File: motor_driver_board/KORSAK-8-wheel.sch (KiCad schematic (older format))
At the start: 24 parts, among them J1 Screw_Terminal_01x04, J2 Conn_01x02_Male, J3 Screw_Terminal_01x06, J4 Screw_Terminal_01x04, M1 Motor_DC, M2 Motor_DC, M3 Motor_DC, M4 Motor_DC, M5 Motor_DC, M6 Motor_DC, M7 Motor_DC, M8 Motor_DC, U1 L293D, U2 L293D, U3 L293D, U4 L293D

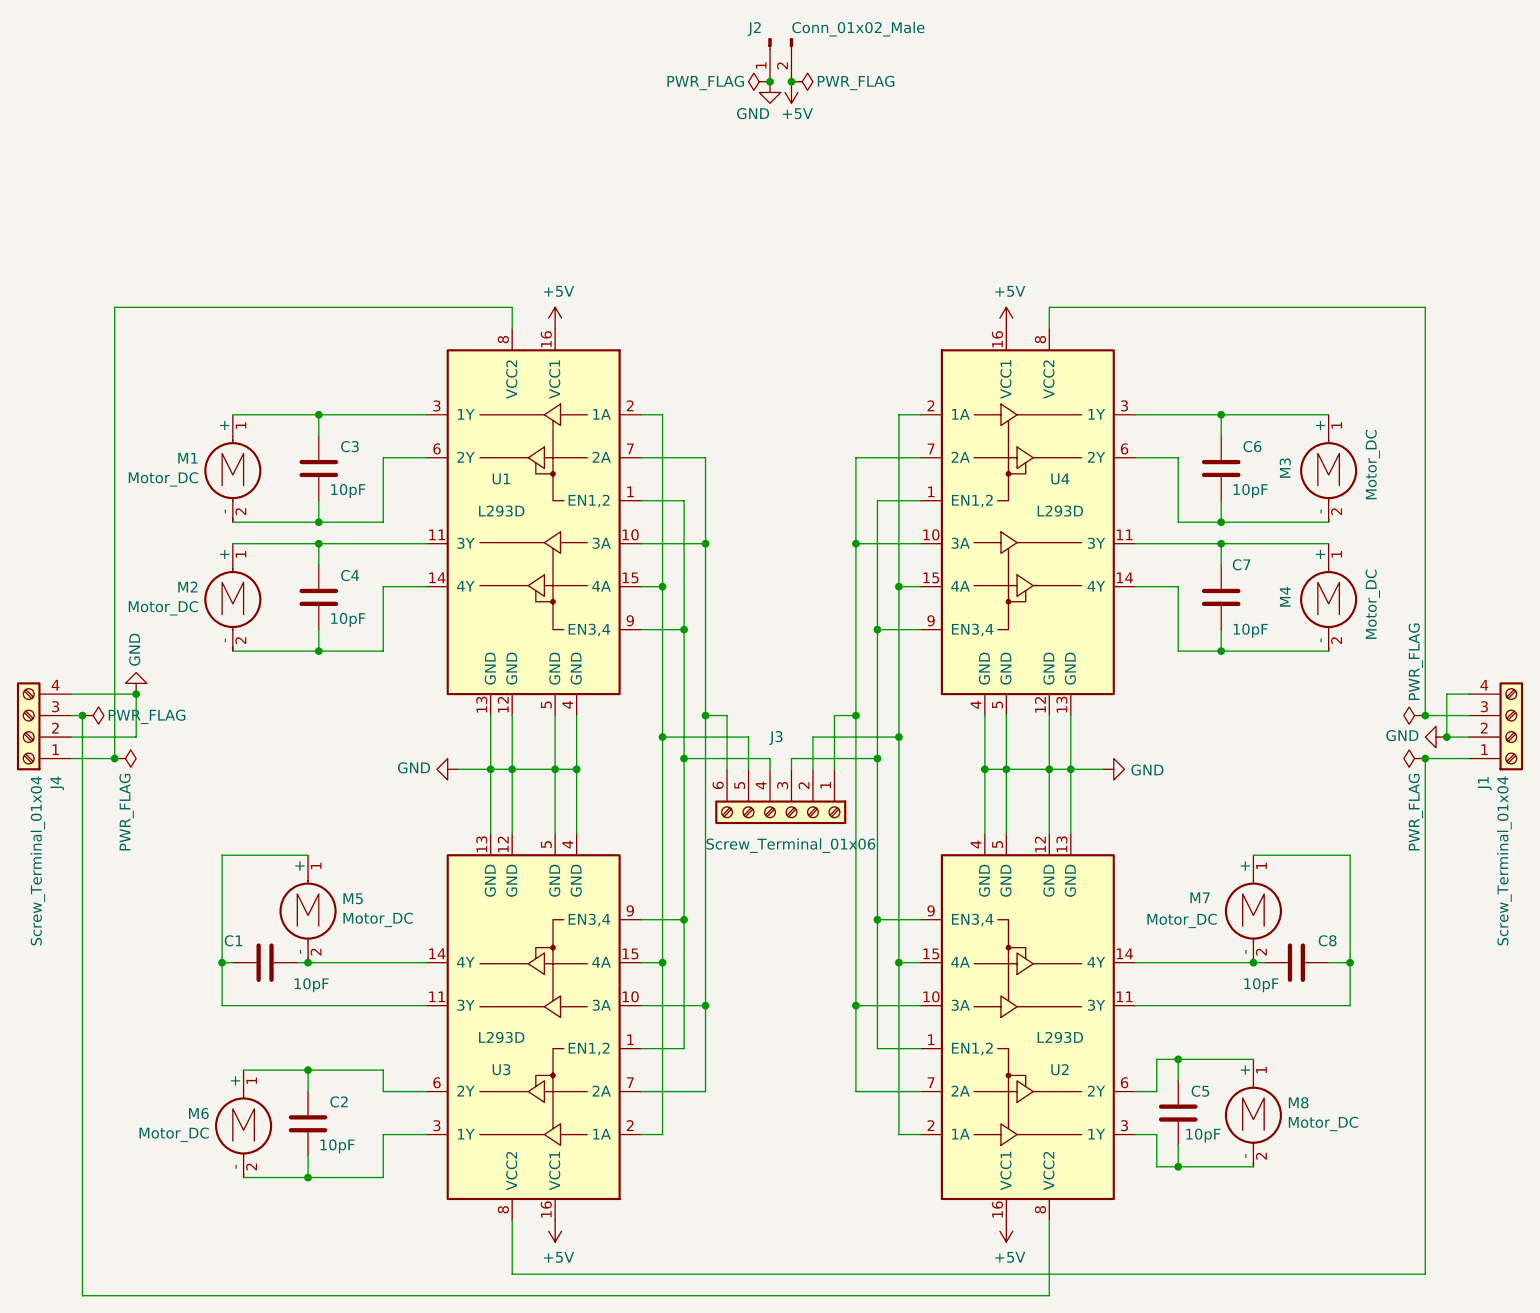
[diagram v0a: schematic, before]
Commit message: Откат прошлого коммита, т.к. это незаконченная версия
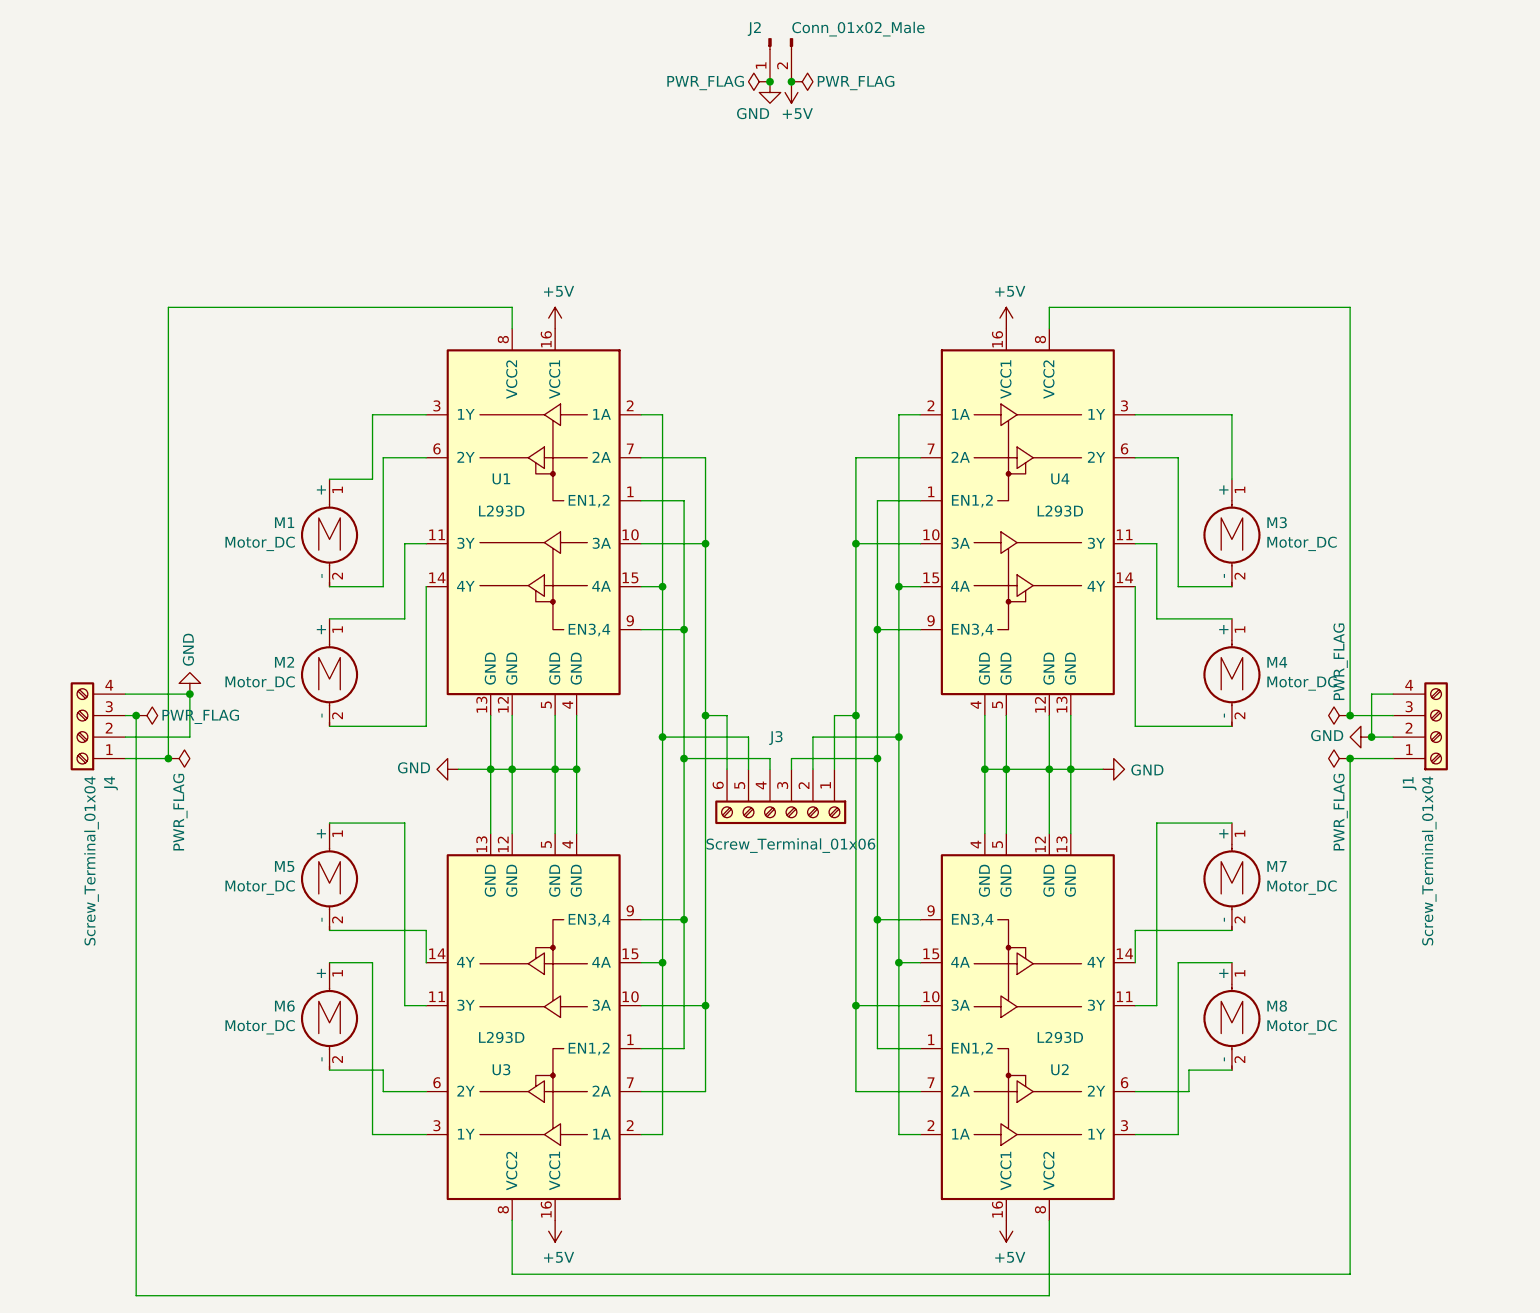
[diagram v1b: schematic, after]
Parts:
- removed C1, C2, C3, C4, C5, C6, C7, C8: 10pF, symbol Device:C
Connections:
- net at M8.1 (+): now also U2.3 (1Y); no longer U2.6 (2Y)
- net at M8.2 (-): now also U2.6 (2Y); no longer U2.3 (1Y)
- net at U3.3 (1Y): now also M6.1 (+); no longer M6.2 (-)
- net at U3.6 (2Y): now also M6.2 (-); no longer M6.1 (+)
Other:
- moved on the sheet: J1, J4, M1, M2, M3, M4, M5, M6, M7, M8
